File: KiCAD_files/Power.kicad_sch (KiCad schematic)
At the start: 62 parts, among them J11 Conn_01x01, J14 Conn_01x01, J17 Conn_01x01, J2 2604-1102, J20 Conn_01x01, J27 Conn_01x01, J28 Conn_01x01, J29 Conn_01x01, J3 Conn_01x01, J30 Conn_01x01, J32 Conn_01x01, J33 Conn_01x01, J34 Conn_01x01, J35 Conn_01x01, J4 2604-1102, J5 2604-1102, U13 OPA316, U3 ACS712xLCTR-20A, U5 AMC1311, U8 OPA316

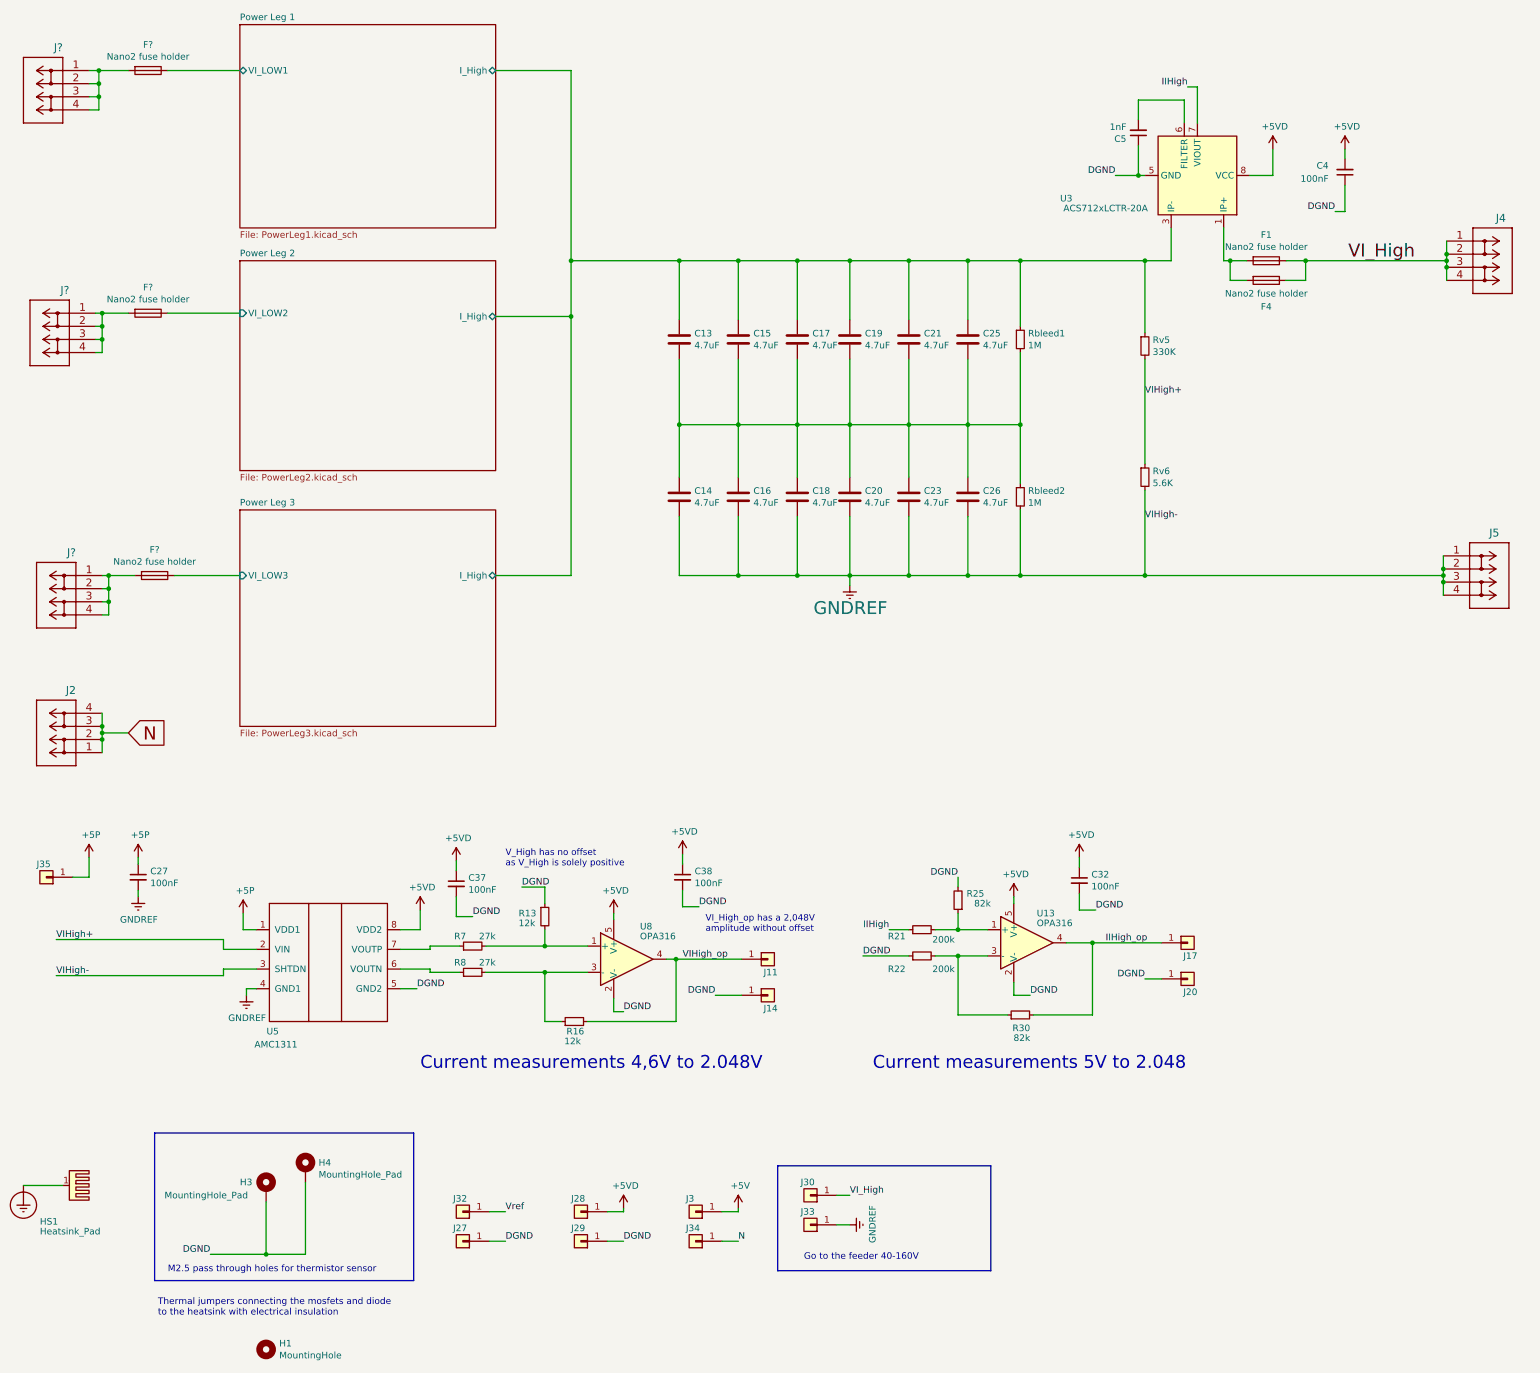
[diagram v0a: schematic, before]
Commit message: Added feeder project alpha version
Former-commit-id: 38773bad2925cccbdf57e9531d71dd427b0662b4
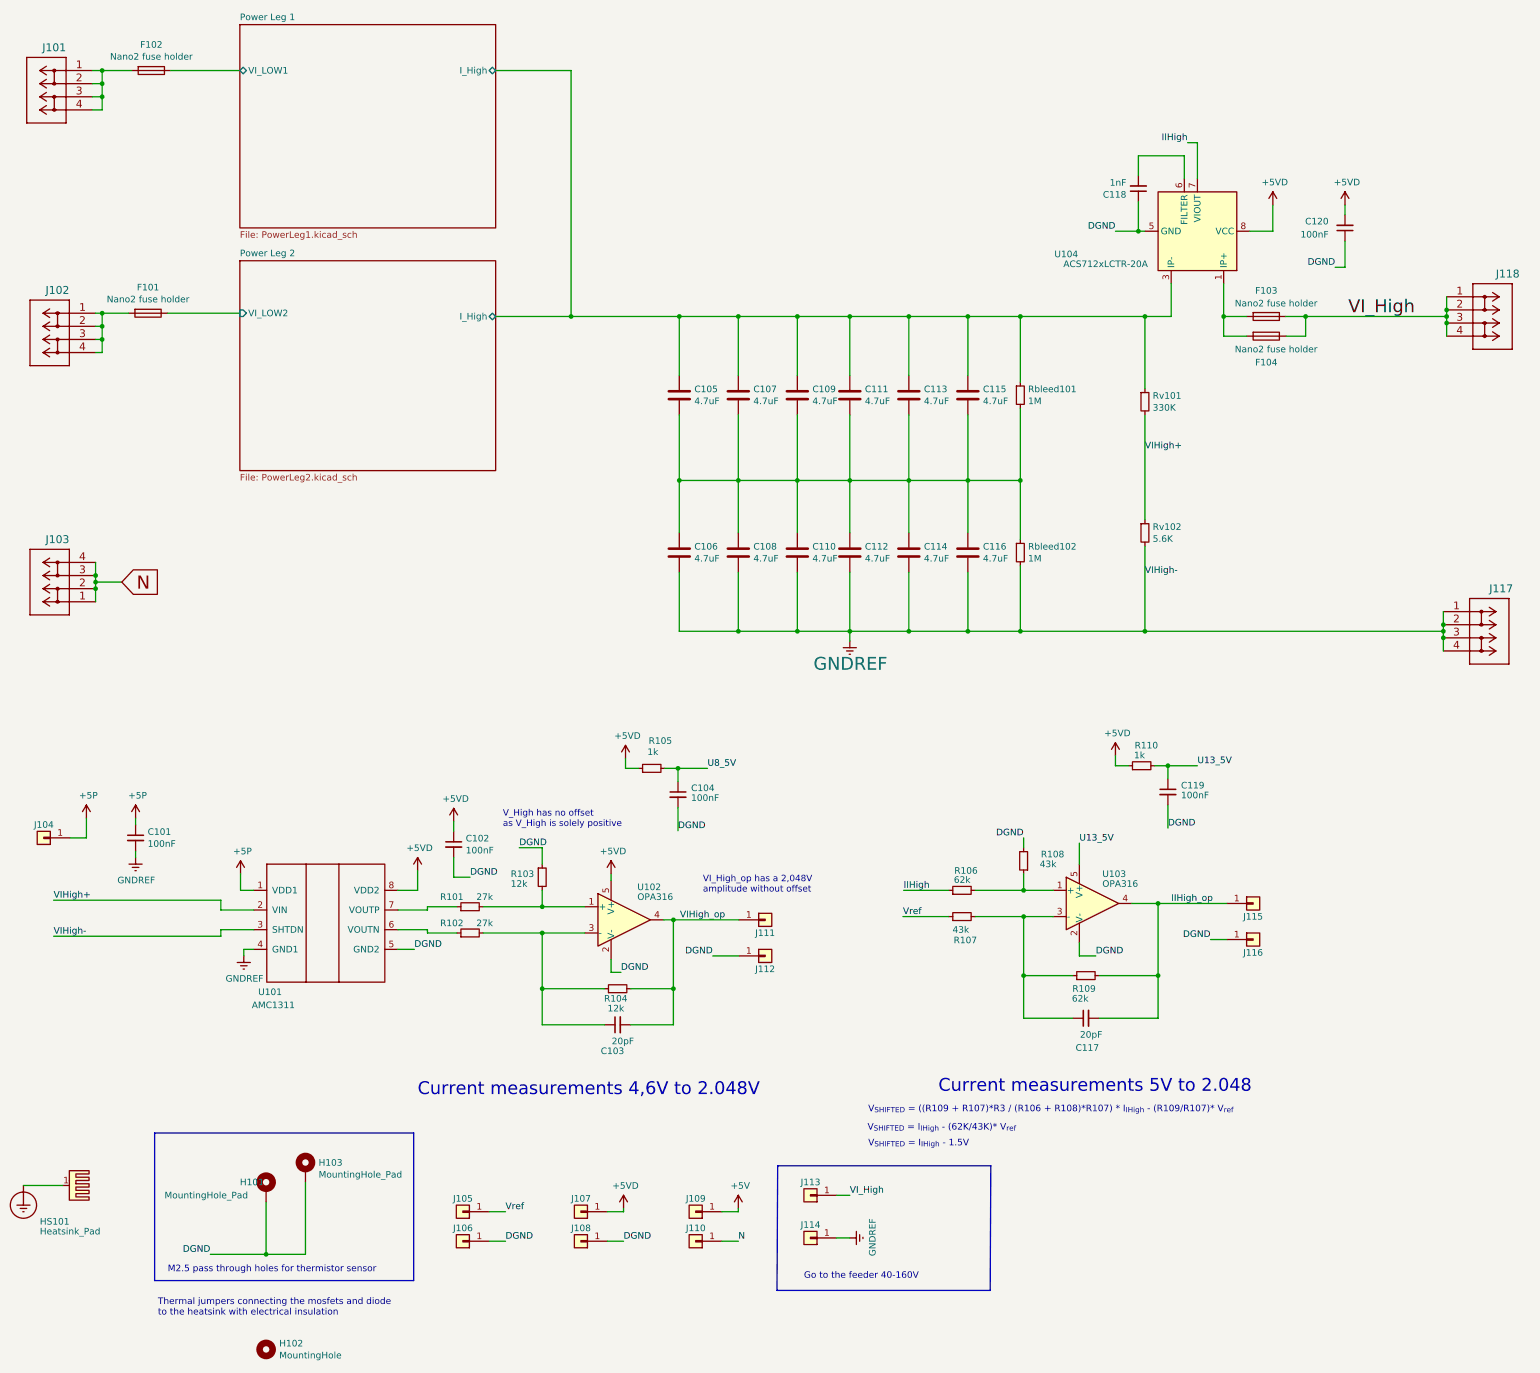
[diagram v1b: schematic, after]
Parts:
- removed C38: 100nF, Capacitor_SMD:C_0805_2012Metric, symbol Device:C_Small
- removed F?: Nano2 fuse holder, Footprints:Fuse_holder_omni_blok, symbol Device:Fuse
- removed J?: 2604-1102, Footprints:WAGO-2604-1102, symbol Symbols:2604-1102
- added C103, C117: 20pF, Capacitor_SMD:C_0805_2012Metric, symbol Device:C_Small
- added C104: 100nF, Capacitor_SMD:C_0805_2012Metric, symbol Device:C_Small
- added R105, R110: 1k, Resistor_SMD:R_0805_2012Metric, symbol Device:R_Small
- R106: renamed from R21; value 200k -> 62k
- R107: renamed from R22; value 200k -> 43k
- R108: renamed from R25; value 82k -> 43k
- R109: renamed from R30; value 82k -> 62k
- gave numbers to parts that had none: 4
- renumbered C27 to C101, C37 to C102, C13 to C105, C14 to C106, C15 to C107, C16 to C108, C17 to C109, C18 to C110, C19 to C111, C20 to C112, C21 to C113, C23 to C114, C25 to C115, C26 to C116, C5 to C118, C32 to C119, C4 to C120, F1 to F103, F4 to F104, H3 to H101, H1 to H102, H4 to H103, HS1 to HS101, J2 to J103, J35 to J104, J32 to J105, J27 to J106, J28 to J107, J29 to J108, J3 to J109, J34 to J110, J11 to J111, J14 to J112, J30 to J113, J33 to J114, J17 to J115, J20 to J116, J5 to J117, J4 to J118, R7 to R101, R8 to R102, R13 to R103, R16 to R104, Rbleed1 to Rbleed101, Rbleed2 to Rbleed102, Rv5 to Rv101, Rv6 to Rv102, U5 to U101, U8 to U102, U13 to U103, U3 to U104
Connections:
- net +5VD: now also R105.1, R110.1; no longer C119.1, U103.5 (V+)
- net DGND: now also C104.2; no longer R107.1
- net IIHigh_op: now also C117.2
- net VIHigh_op: now also C103.2
- net Vref: now also R107.1
- net at R107.2, R109.1, U103.3 (-): now also C117.1
- net at R102.2, R104.1, U102.3 (-): now also C103.1
- new net U13_5V: C119.1, R110.2, U103.5 (V+)
- new net U8_5V: C104.1, R105.2
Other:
- removed sheet Power Leg 3
- note added: "V_{SHIFTED} = ((R109 + R107)*R3 / (R106 + R108)*R107) * I_{IHigh} - (R109/R107)* V_{ref}"
- note added: "V_{SHIFTED} = I_{IHigh} - (62K/43K)* V_{ref}"
- note added: "V_{SHIFTED} = I_{IHigh} - 1.5V"
- moved on the sheet: C101, C102, C105, C106, C107, C108, C109, C110, C111, C112, C113, C114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

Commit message: WIP routing the power board
Former-commit-id: fec71ccccc2062c429ca6048755d91568543f1a5
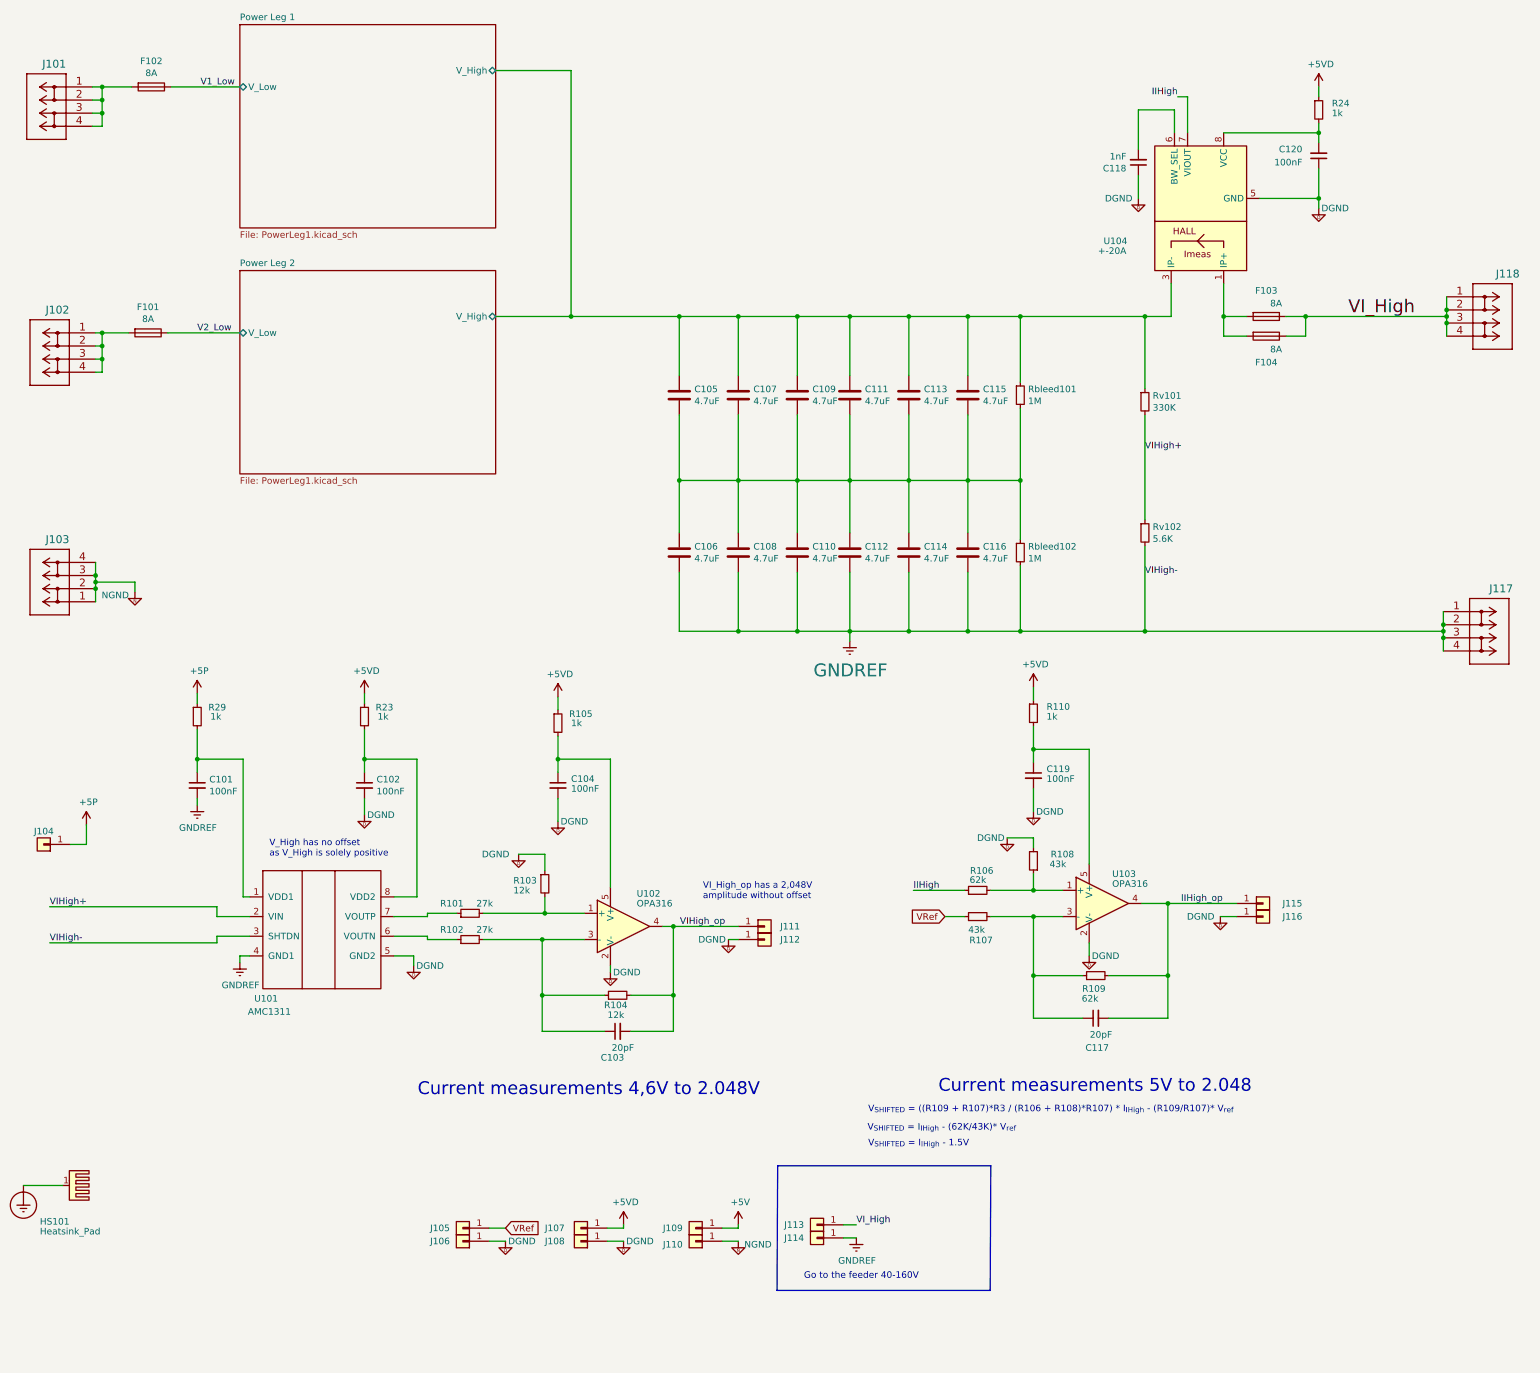
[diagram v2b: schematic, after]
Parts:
- removed H101, H103: MountingHole_Pad, MountingHole:MountingHole_2.2mm_M2_ISO7380_Pad, symbol Mechanical:MountingHole_Pad
- removed H102: MountingHole, Footprints:mounting_holes, symbol Mechanical:MountingHole
- added R23, R24, R29: 1k, Resistor_SMD:R_0805_2012Metric, symbol Device:R_Small
- F101, F102, F103, F104: value Nano2 fuse holder -> 8A
- U101: footprint Footprints:SOIC-8_7.5x5.85mm_P1.27mm -> Package_SO:SOIC-8_7.5x5.85mm_P1.27mm
- U104: value ACS712xLCTR-20A -> +-20A; symbol Sensor_Current:ACS712xLCTR-20A -> Symbols:ACS723
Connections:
- net +5P: now also R29.1; no longer C101.1, U101.1 (VDD1)
- net +5VD: now also R23.1, R24.1; no longer C102.1, C120.2, U101.8 (VDD2), U102.5 (V+), U104.8 (VCC)
- net N renamed NGND
- net Power Leg 1/I_High renamed Power Leg 1/V_High
- net Power Leg 1/VI_LOW1 renamed V1_Low
- net Power Leg 2/VI_LOW2 renamed V2_Low
- net U13_5V: no longer names the net of C119.1, R110.2, U103.5 (V+)
- net U8_5V: no longer names the net of C104.1, R105.2
- net U8_5V: now also U102.5 (V+)
- net Vref renamed VRef
- new net: C120.2, R24.2, U104.8 (VCC)
- new net: C101.1, R29.2, U101.1 (VDD1)
- new net: C102.1, R23.2, U101.8 (VDD2)
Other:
- sheet Power Leg 1 ports: added V_High, V_Low; removed I_High, VI_LOW1
- sheet Power Leg 2: file PowerLeg2.kicad_sch -> PowerLeg1.kicad_sch
- sheet Power Leg 2 ports: added V_High, V_Low; removed I_High, VI_LOW2
- note removed: "M2.5 pass through holes for thermistor sensor"
- note removed: "Thermal jumpers connecting the mosfets and diode to the heatsink with electrical insulation"
- moved on the sheet: C101, C102, C103, C104, C117, C118, C119, C120, F101, F102, J101, J102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
